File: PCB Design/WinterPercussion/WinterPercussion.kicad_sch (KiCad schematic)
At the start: 7 parts, among them J1 SDS-50J, U1 6N138, U2 ESP32-DevKitC

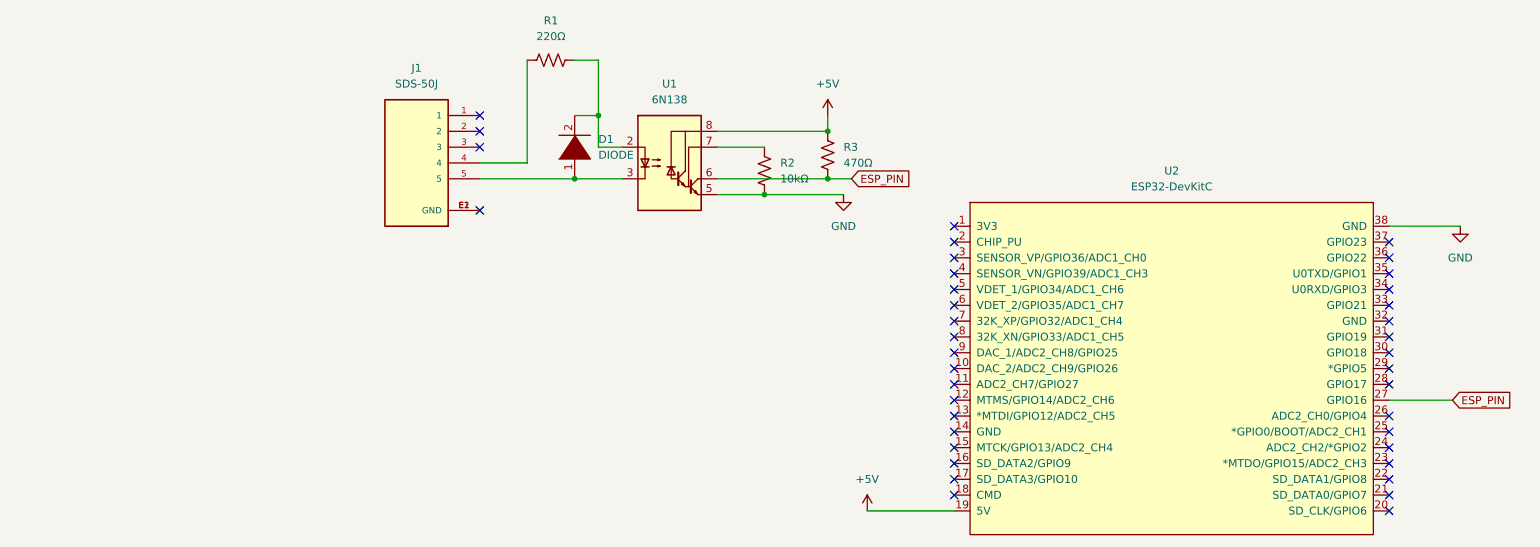
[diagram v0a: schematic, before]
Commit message: Updated KiCad Docs
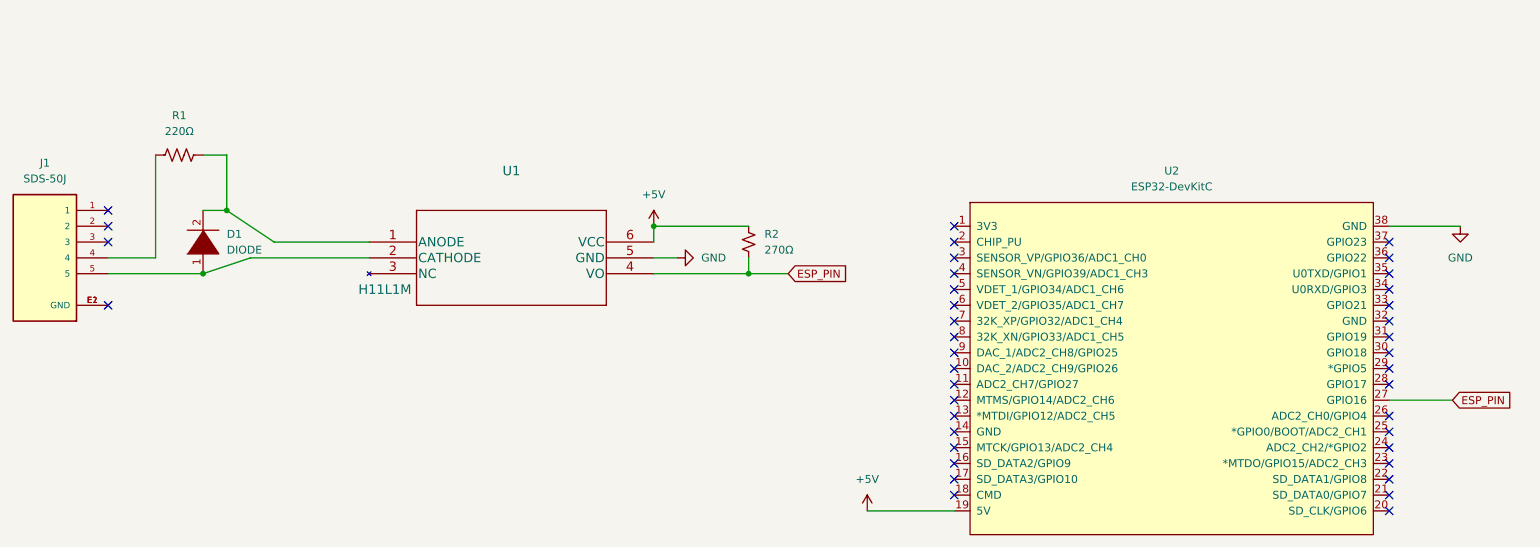
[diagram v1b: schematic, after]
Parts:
- removed R2: 10kΩ, Resistor_THT:R_Axial_DIN0207_L6.3mm_D2.5mm_P7.62mm_Horizontal, symbol Device:R_US
- removed R3: 470Ω, Resistor_THT:R_Axial_DIN0207_L6.3mm_D2.5mm_P7.62mm_Horizontal, symbol Device:R_US
- removed U1: 6N138, OptoCoupler:DIP762W50P254L1018H450Q8, symbol Isolator:6N138
- added R2: 270Ω, Resistor_THT:R_Axial_DIN0207_L6.3mm_D2.5mm_P7.62mm_Horizontal, symbol Device:R_Small_US
- added U1: H11L1M, Opto:H11L1M, symbol OptoCoupler:H11L1M
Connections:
- net +5V: now also R2.1, U1.6 (VCC)
- net ESP_PIN: now also R2.2, U1.4 (VO)
- net GND: now also U1.5 (GND)
- net at D1.2 (A), R1.1: now also U1.1 (ANODE)
- net at D1.1 (K), J1.5: now also U1.2 (CATHODE)
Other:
- moved on the sheet: D1, J1, R1
